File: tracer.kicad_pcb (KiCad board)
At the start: 4 copper layers, 22 x 45 mm, 19 parts, among them J1 IO_JACK_F04_SPLIT, K1 Coto-9913-05-20, K2 Coto-9913-05-20, Q1 MMBT3904, Q2 MMBT3904, U1 AD8403ARZ1, U2 AD8403ARZ1, U3 TXS0101

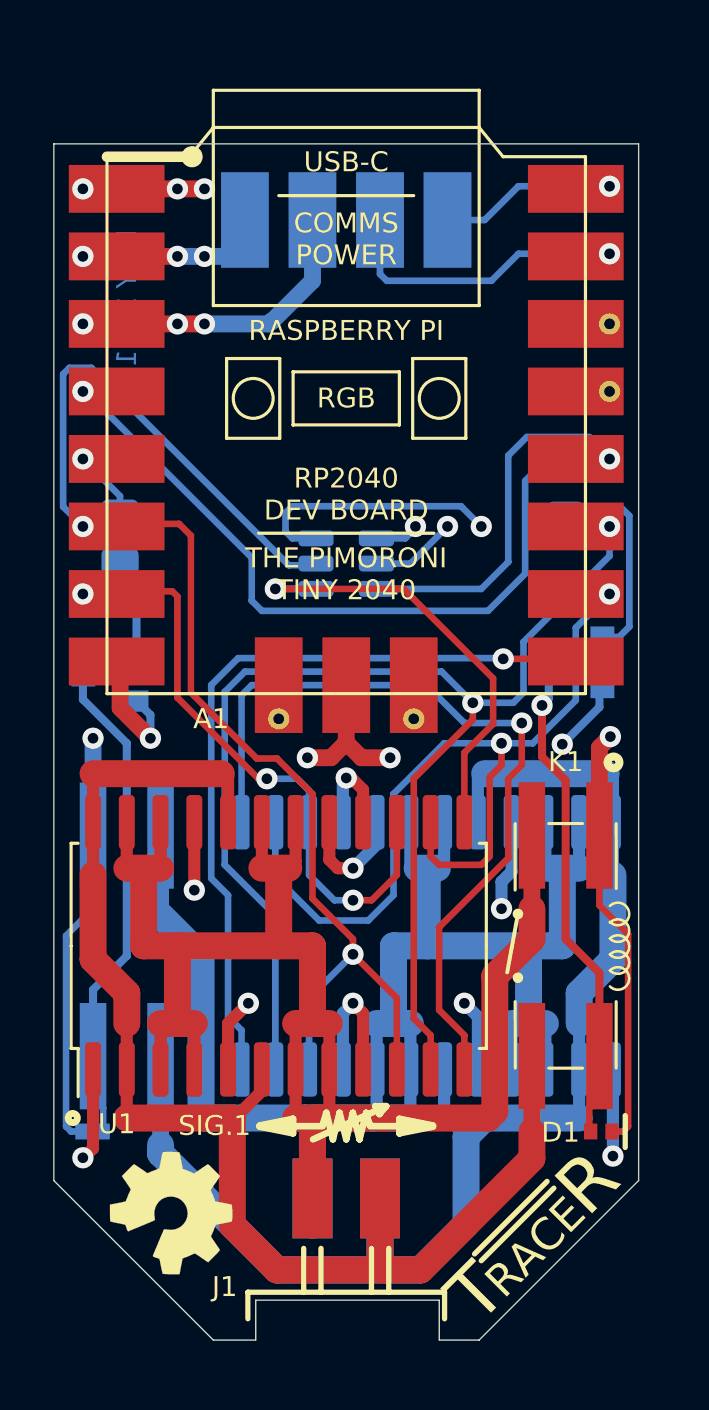
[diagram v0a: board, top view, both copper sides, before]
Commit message: v2 release to PCB shop
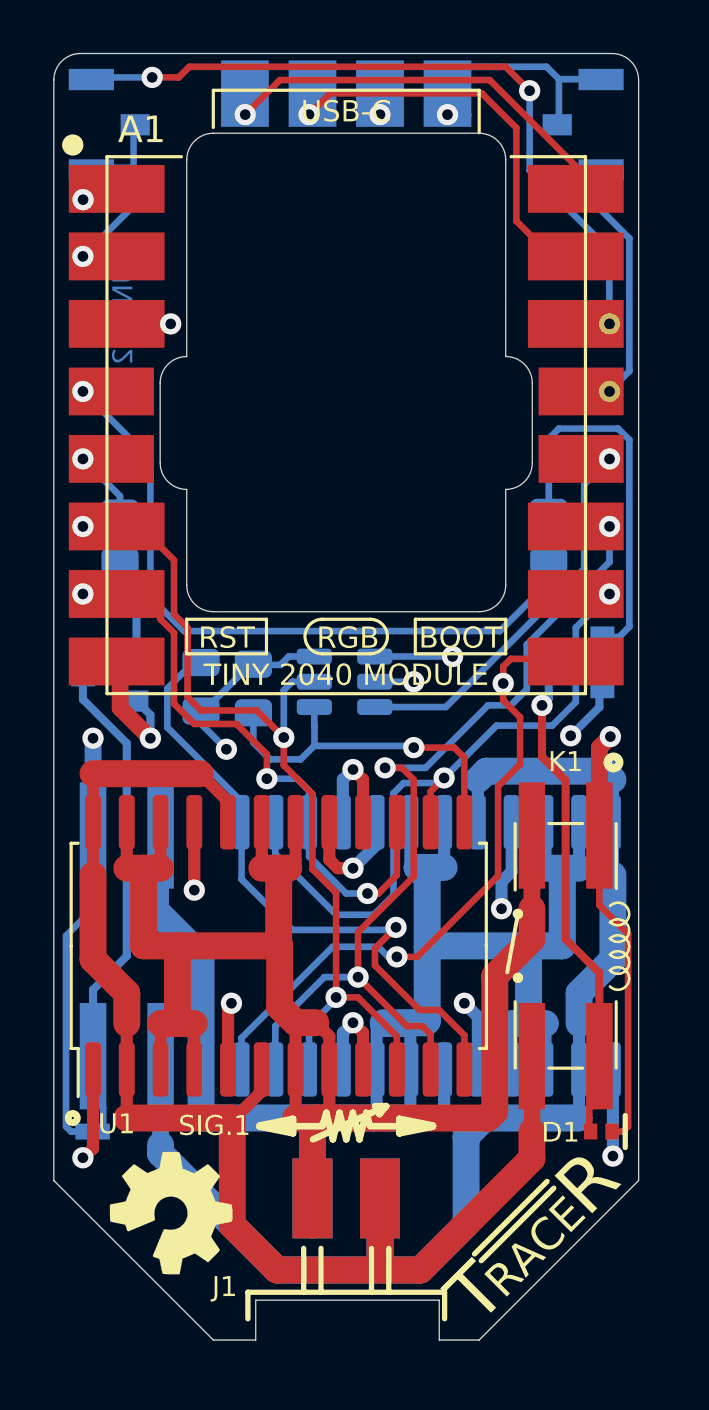
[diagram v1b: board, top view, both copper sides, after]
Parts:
- removed TP17, TP19: TestPoint, .tracer:via-0.8x0.4
- added R3: 1K, .tracer:R_0805_2012Metric, B.Cu at (-3.49, -24.5)
- added R4: 1K, .tracer:R_0805_2012Metric, B.Cu at (-5.46, -24.6)
- added S1: B3U-3100P-B, .tracer:SW_B3U-3100P-B, B.Cu at (9.59, -45.7)
- added S2: B3U-3100P-B, .tracer:SW_B3U-3100P-B, B.Cu at (-9.59, -45.7)
- A1: footprint .tracer:MODULE_TINY_2040 -> .tracer:MODULE_TINY_2040_DEV2
- A2: footprint .tracer:MODULE_OLED_490 -> .tracer:MODULE_OLED_490_SMALL_PADS
- moved A2 4.75 mm to (0.00, -46.0)
- moved U3 4.45 mm to (-0.06, -24.8)
- moved R1 1.83 mm to (7.62, -30.2), turned to 270 degrees
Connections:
- A2 pad 1: Net-(A1-Pad16) -> GND
- A2 pad 2: Net-(A1-Pad15) -> +3V3
- A2 pad 3: +3V3 -> Net-(A1-Pad15)
- A2 pad 4: GND -> Net-(A1-Pad16)
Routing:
- net Net-(A1-Pad14): track 0.00 -> 27.1 mm, vias 0 -> 2
- net /~SHDN: track 51.7 -> 34.5 mm, vias 2 -> 3
- net /~SS: track 49.8 -> 34.0 mm, vias 2 -> 3
- net Net-(A1-Pad16): track 6.62 -> 16.0 mm
- net Net-(A1-Pad13): track 0.00 -> 9.06 mm
- net +3V3: track 13.2 -> 5.81 mm, vias 4 -> 3
- net /CLK: track 32.4 -> 25.5 mm
- net +5V: track 50.3 -> 43.5 mm, vias 7 -> 5
- net Net-(Q1-Pad1): track 8.03 -> 14.2 mm
- net /SDO2: track 30.8 -> 25.0 mm
- net Net-(A1-Pad15): track 11.2 -> 15.8 mm
- net /SDI: track 29.1 -> 25.1 mm, vias 1 -> 2
- net /SDO1_5V: track 17.1 -> 13.7 mm
- net GND: track 56.3 -> 54.6 mm, vias 16 -> 13
- net /SIG2A: track 62.2 -> 63.3 mm
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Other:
- board size 22 x 45 mm -> 22 x 48.4 mm
- net class Default: clearance 0.2 -> 0.19
- rule trace_clearance: 0.2 -> 0.19
- board text added: "V2 JUN 2021"
- board text removed: "V2 MAY 2021"
